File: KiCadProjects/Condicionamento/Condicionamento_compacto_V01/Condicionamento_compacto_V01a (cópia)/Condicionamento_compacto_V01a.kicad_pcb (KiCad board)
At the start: 2 copper layers, 45 x 25 mm, 19 parts, among them J1 Entrada, J2 Canais, J3 Conn_01x03, J4 Conn_01x03, U1-Cond1 AD828AN

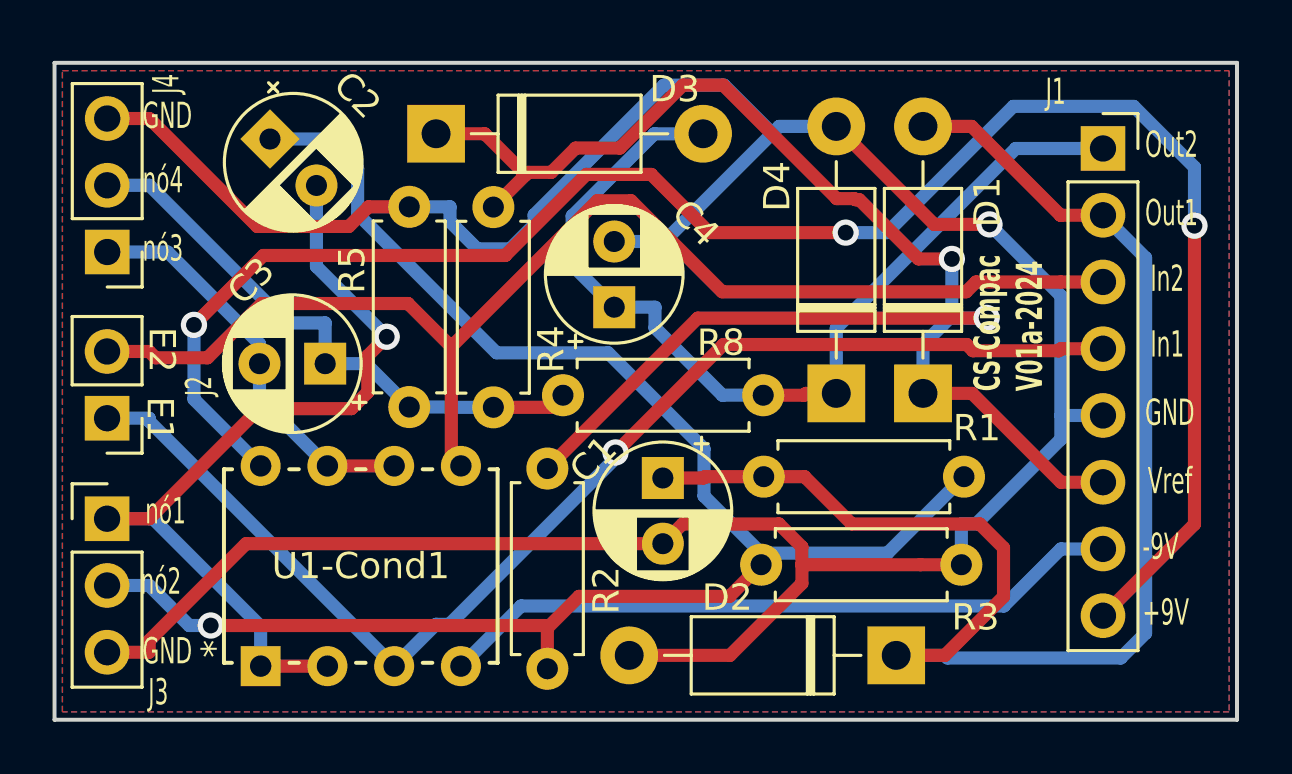
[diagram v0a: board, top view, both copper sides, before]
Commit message: enviar para producao
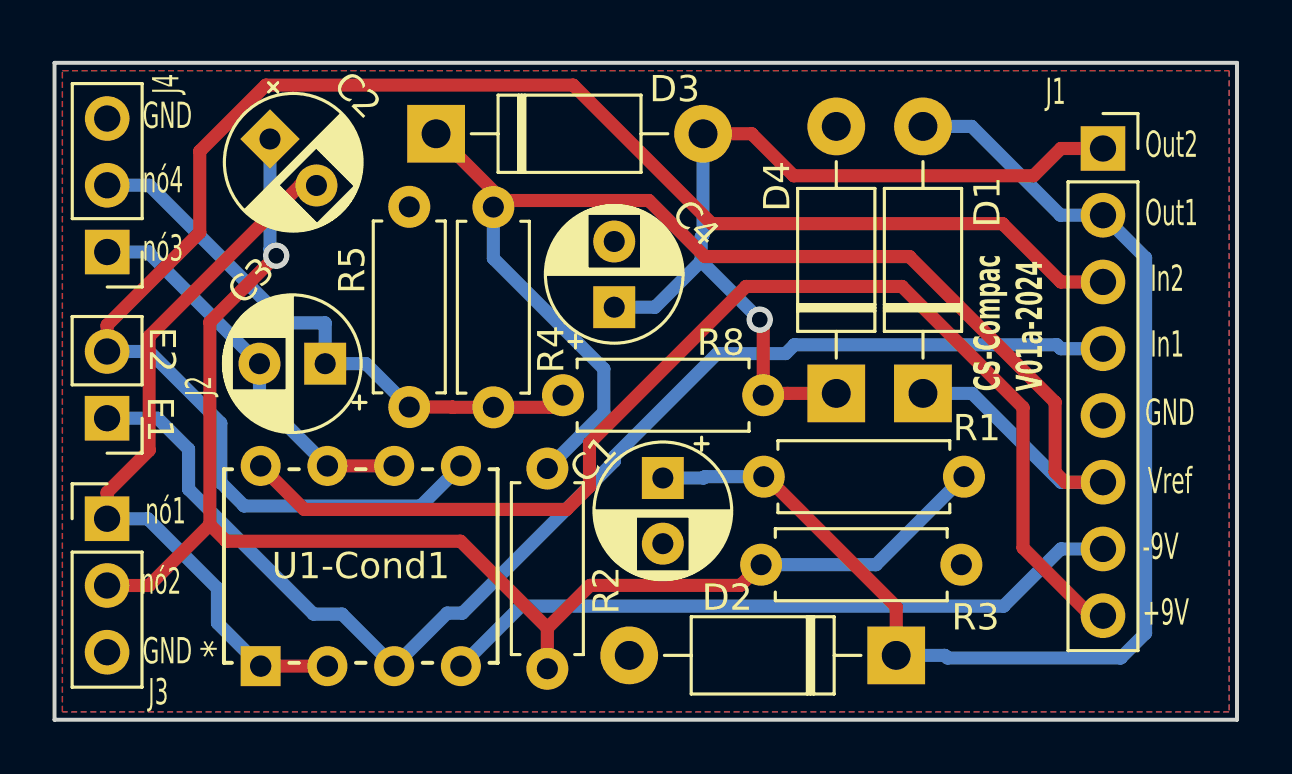
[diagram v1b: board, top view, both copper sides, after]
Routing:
- net Earth: track 111.3 -> 0.00 mm, vias 1 -> 0
- net +9V: track 69.2 -> 45.5 mm, vias 3 -> 0
- net Canal_2: track 48.1 -> 65.5 mm
- net nó2: track 64.8 -> 55.0 mm
- net Out_1: track 55.7 -> 47.6 mm
- net Vref: track 60.5 -> 53.7 mm, vias 2 -> 0
- net nó1: track 32.8 -> 27.8 mm, vias 1 -> 0
- net Out_2: track 36.2 -> 34.1 mm, vias 0 -> 1
- net Canal_1: track 47.2 -> 47.9 mm, vias 1 -> 0
